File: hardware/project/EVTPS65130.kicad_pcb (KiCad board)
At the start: 2 copper layers, 32 x 34.4 mm, 53 parts, among them J1 USB_C_Receptacle_PowerOnly_6P, J2 Conn_01x04_Pin, Q10 PMOS, U3 TPS65130RGE

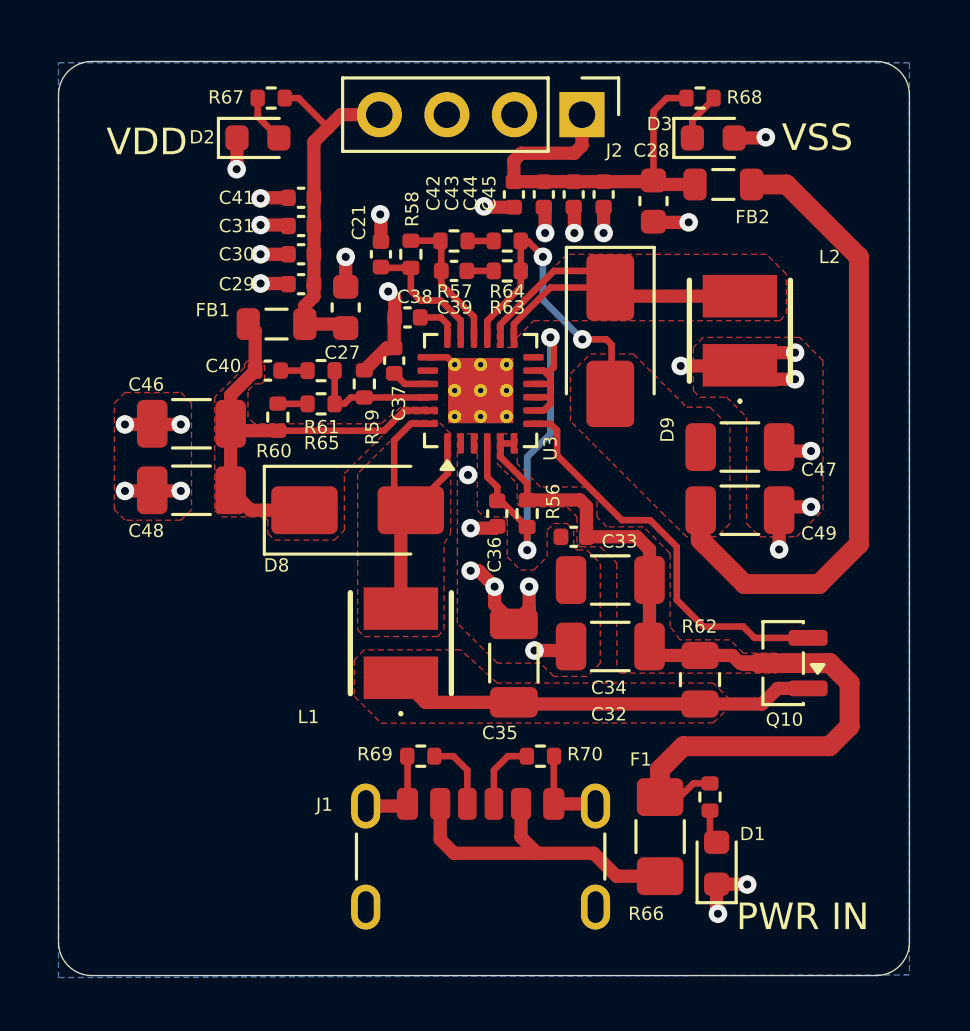
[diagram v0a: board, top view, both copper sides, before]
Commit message: Revert "Finished PCB"
This reverts commit 62ccf1f0346de98fa26003fa6e9ccd42f55a9d01.
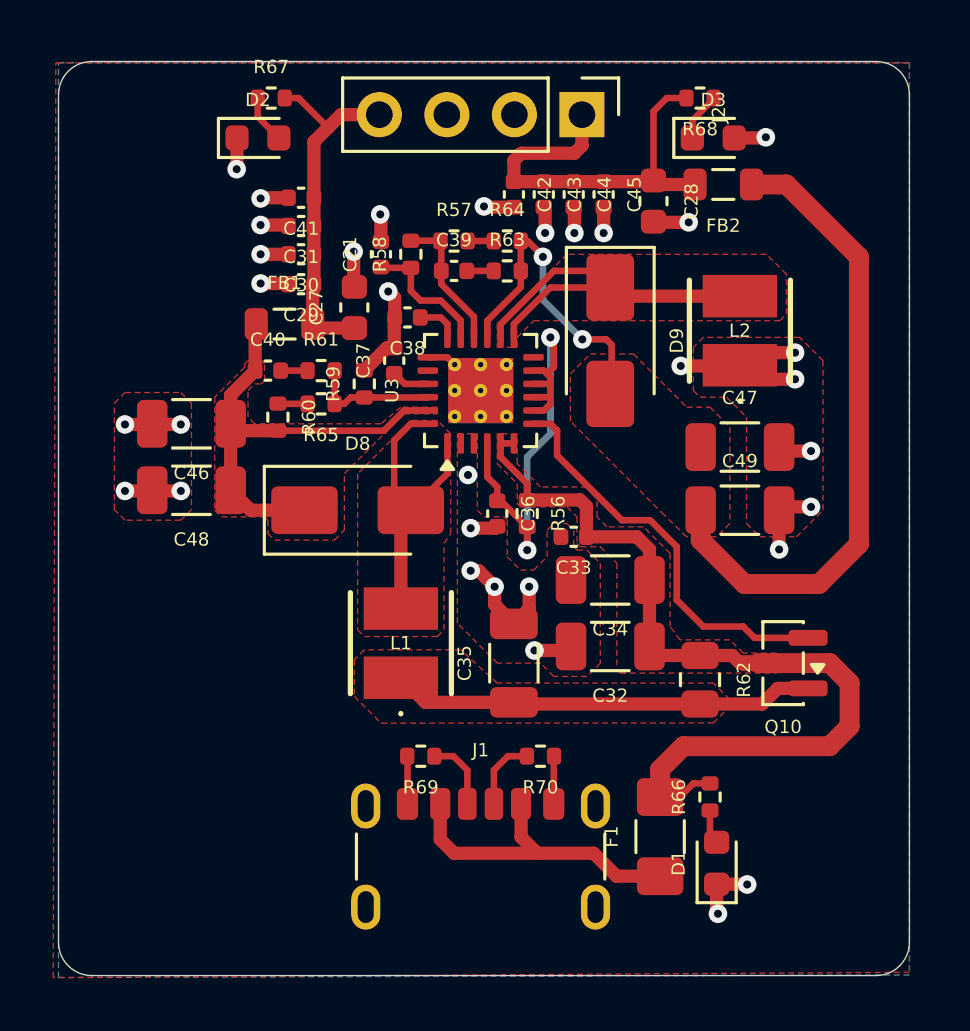
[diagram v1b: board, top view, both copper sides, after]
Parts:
- moved C27 0.32 mm to (139.6, 120.0)
- moved FB1 0.30 mm to (137.0, 120.6)
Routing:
- net AGND: track 50.2 -> 47.2 mm
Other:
- board text removed: "PWR IN"
- board text removed: "VDD"
- board text removed: "VSS"

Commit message: Finished PCB
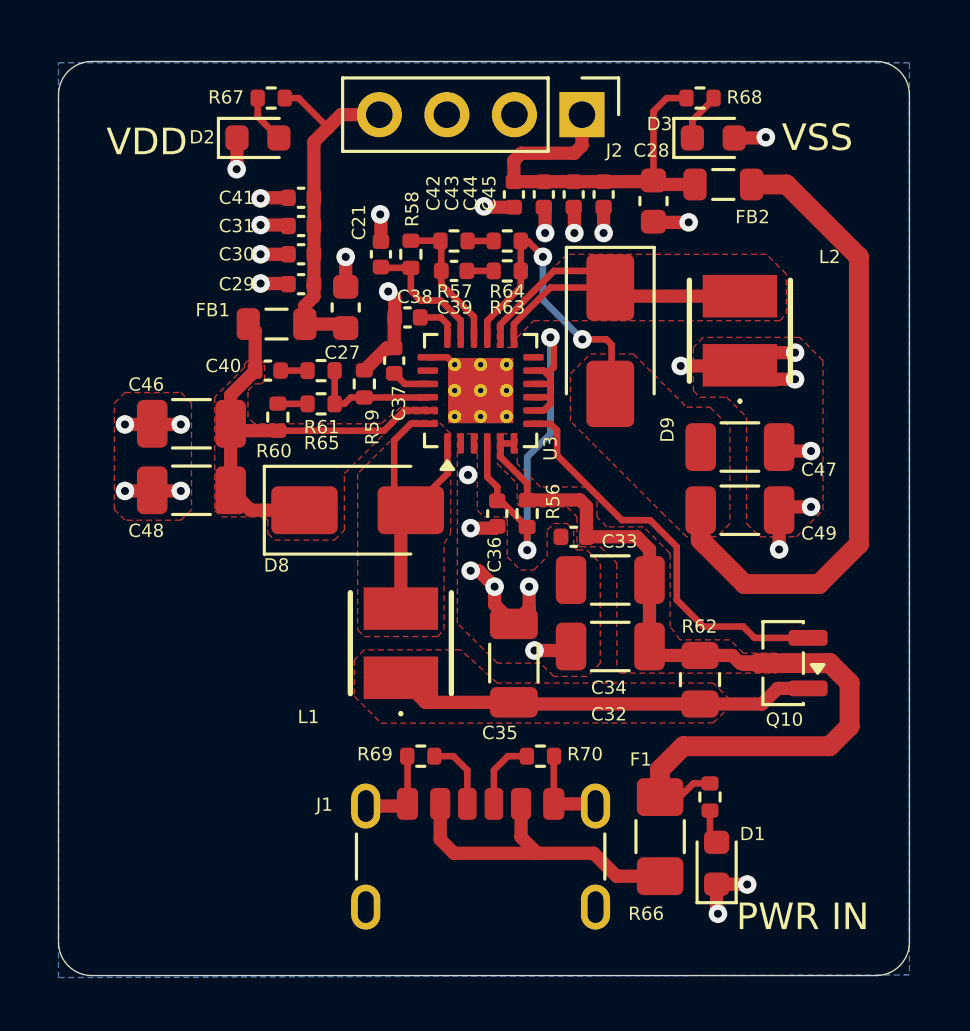
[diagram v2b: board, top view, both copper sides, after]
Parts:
- moved C27 0.32 mm to (139.3, 120.0)
- moved FB1 0.30 mm to (136.7, 120.6)
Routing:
- net AGND: track 47.2 -> 50.2 mm
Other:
- board text added: "PWR IN"
- board text added: "VDD"
- board text added: "VSS"
